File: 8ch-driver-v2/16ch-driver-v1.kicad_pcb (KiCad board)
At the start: 4 copper layers, 191.8 x 156.5 mm, 233 parts, among them J1 Barrel_Jack, Q1 2N7002E, Q10 2N7002E, Q11 2N7002E, Q12 2N7002E, Q13 2N7002E, Q14 2N7002E, Q15 2N7002E, Q16 2N7002E, Q2 2N7002E, Q3 2N7002E, Q4 2N7002E, Q5 2N7002E, Q6 2N7002E, Q7 2N7002E, Q8 2N7002E, Q9 2N7002E, U1 DRV104PWP, U10 DRV104PWP, U11 DRV104PWP, U12 DRV104PWP, U13 DRV104PWP, U14 DRV104PWP, U15 DRV104PWP, U16 DRV104PWP, U17 BD33FC0FP, U18 FT4232H MINI MODULE, U2 DRV104PWP, U3 DRV104PWP, U4 DRV104PWP, U5 DRV104PWP, U6 DRV104PWP, U7 DRV104PWP, U8 DRV104PWP, U9 DRV104PWP

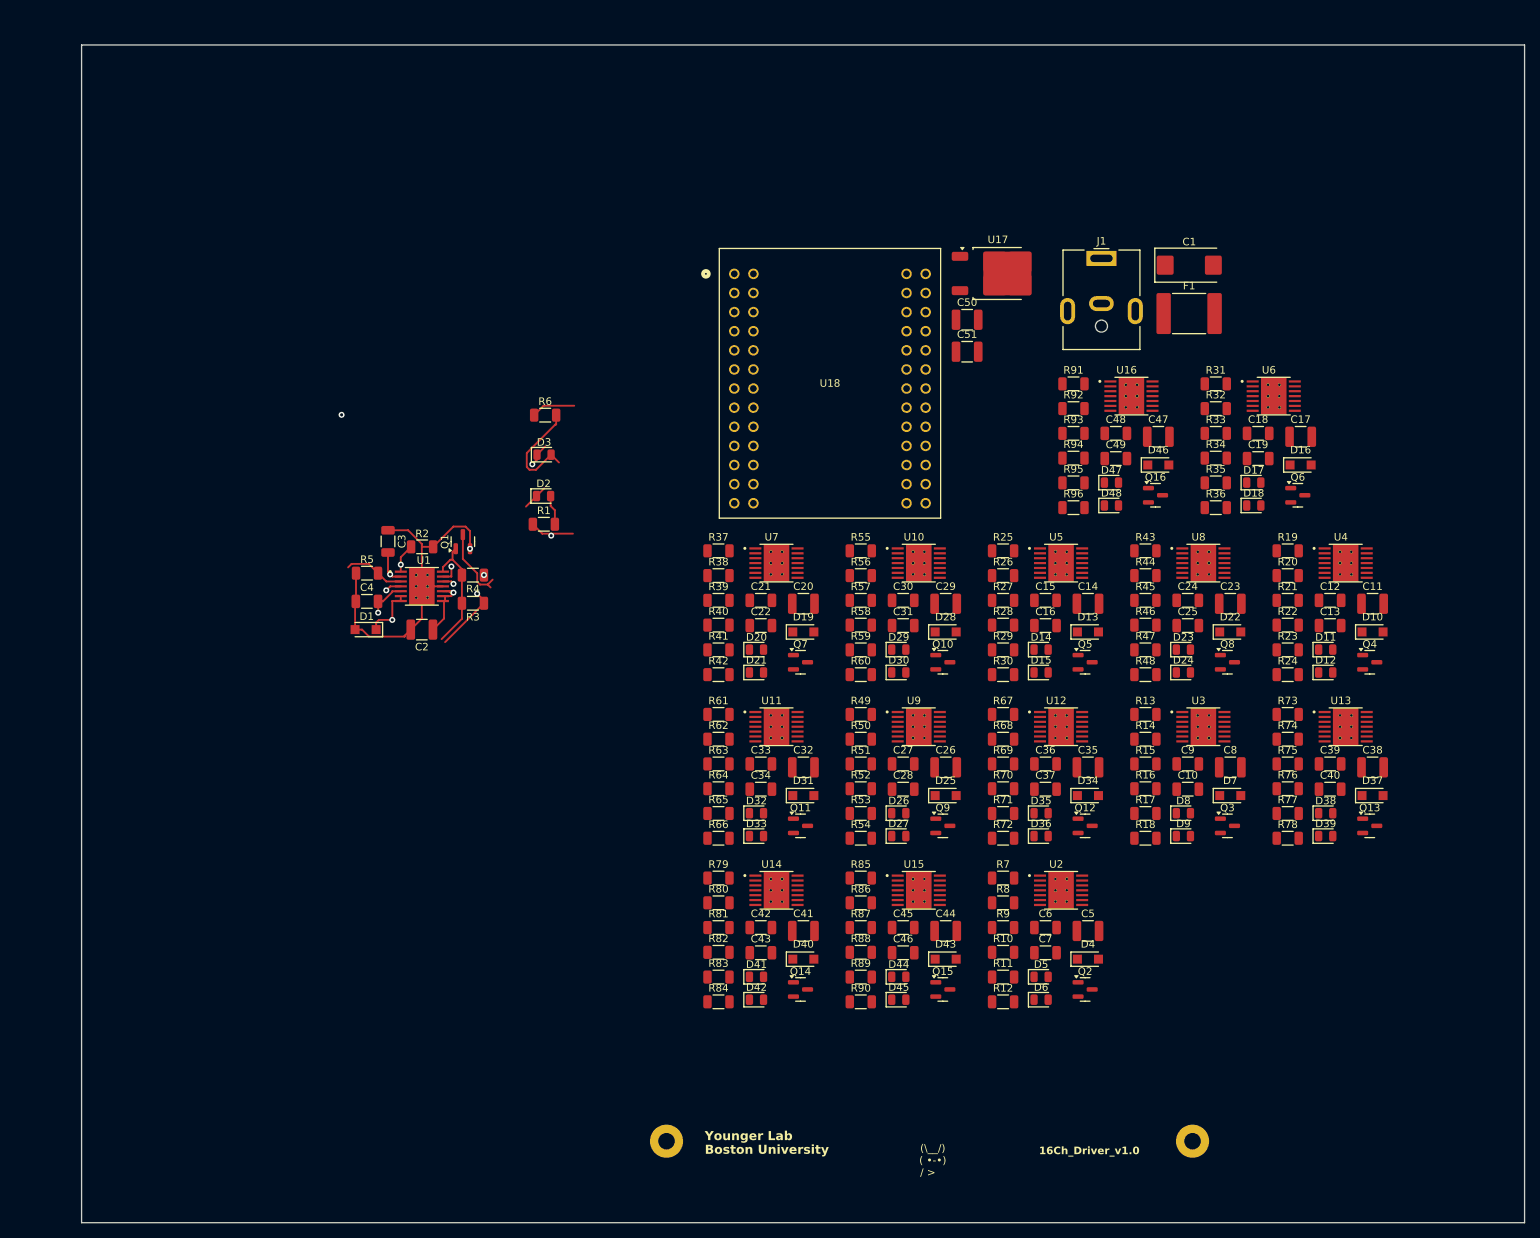
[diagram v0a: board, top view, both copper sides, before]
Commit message: push
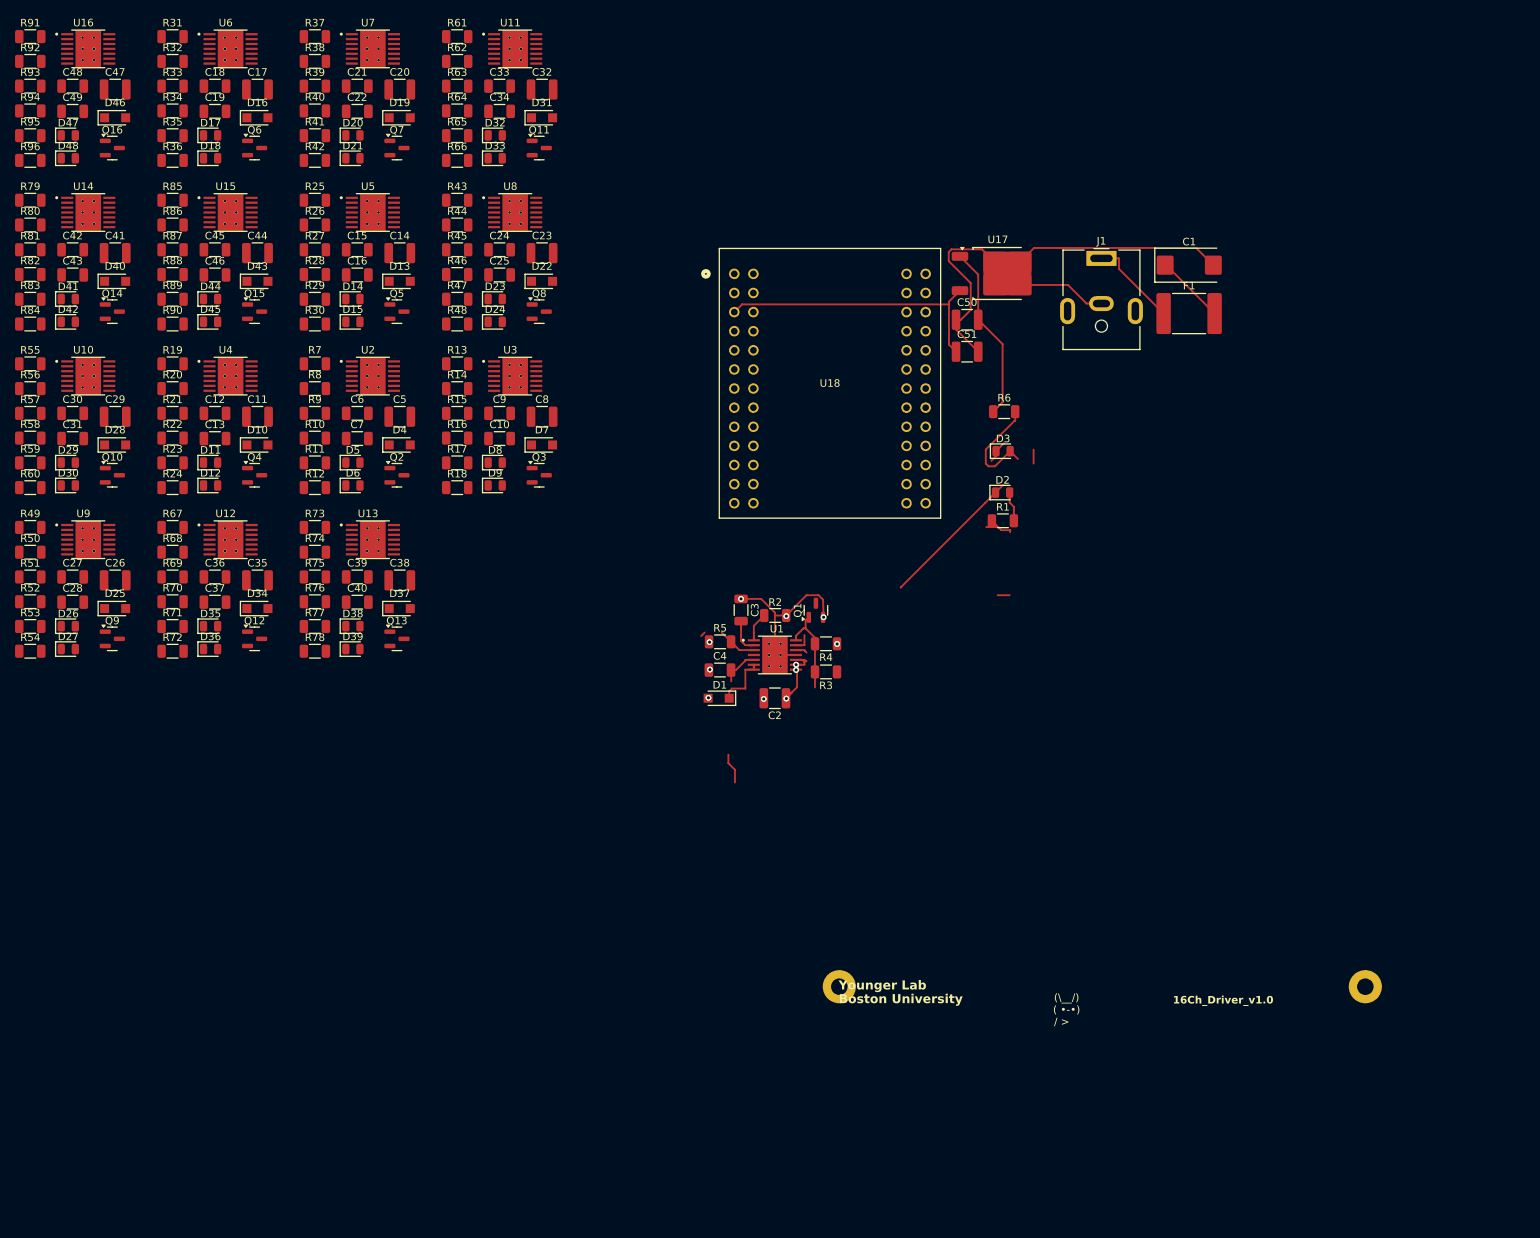
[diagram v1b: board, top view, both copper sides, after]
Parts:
- moved C11 150.2 mm to (46.4, 61.7)
- moved C12 150.2 mm to (40.7, 61.3)
- moved C13 150.2 mm to (40.7, 64.6)
- moved D10 150.2 mm to (46.4, 65.5)
- moved Q4 150.2 mm to (46.0, 69.5)
- moved R19 150.2 mm to (35.1, 54.7)
- moved R20 150.2 mm to (35.1, 58.0)
- moved R21 150.2 mm to (35.1, 61.3)
- moved R22 150.2 mm to (35.1, 64.5)
- moved R23 150.2 mm to (35.1, 67.8)
- moved R24 150.2 mm to (35.1, 71.1)
- moved U4 150.2 mm to (42.8, 56.3)
- moved D11 150.2 mm to (40.1, 67.8)
- moved D12 150.2 mm to (40.1, 70.8)
- moved C17 146.1 mm to (46.4, 18.2)
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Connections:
- net /SpikeAndHoldDriverAndLEDs-1/delay03 renamed /SpikeAndHoldDriverAndLEDs-1/delay
- net /SpikeAndHoldDriverAndLEDs-1/duty03 renamed /SpikeAndHoldDriverAndLEDs-1/duty
- net /SpikeAndHoldDriverAndLEDs-1/fault03 renamed /SpikeAndHoldDriverAndLEDs-1/fault
- net /SpikeAndHoldDriverAndLEDs-1/freq03 renamed /SpikeAndHoldDriverAndLEDs-1/freq
- net /SpikeAndHoldDriverAndLEDs-1/in_term03 renamed Net-(Q1-G)
- net /SpikeAndHoldDriverAndLEDs-10/delay03 renamed /SpikeAndHoldDriverAndLEDs-10/delay
- net /SpikeAndHoldDriverAndLEDs-10/duty03 renamed /SpikeAndHoldDriverAndLEDs-10/duty
- net /SpikeAndHoldDriverAndLEDs-10/fault03 renamed /SpikeAndHoldDriverAndLEDs-10/fault
- net /SpikeAndHoldDriverAndLEDs-10/freq03 renamed /SpikeAndHoldDriverAndLEDs-10/freq
- net /SpikeAndHoldDriverAndLEDs-10/in_term03 renamed Net-(Q10-G)
- net /SpikeAndHoldDriverAndLEDs-11/delay03 renamed /SpikeAndHoldDriverAndLEDs-11/delay
- net /SpikeAndHoldDriverAndLEDs-11/duty03 renamed /SpikeAndHoldDriverAndLEDs-11/duty
- net /SpikeAndHoldDriverAndLEDs-11/fault03 renamed /SpikeAndHoldDriverAndLEDs-11/fault
- net /SpikeAndHoldDriverAndLEDs-11/freq03 renamed /SpikeAndHoldDriverAndLEDs-11/freq
- net /SpikeAndHoldDriverAndLEDs-11/in_term03 renamed Net-(Q11-G)
- net /SpikeAndHoldDriverAndLEDs-12/delay03 renamed /SpikeAndHoldDriverAndLEDs-12/delay
- net /SpikeAndHoldDriverAndLEDs-12/duty03 renamed /SpikeAndHoldDriverAndLEDs-12/duty
- net /SpikeAndHoldDriverAndLEDs-12/fault03 renamed /SpikeAndHoldDriverAndLEDs-12/fault
- net /SpikeAndHoldDriverAndLEDs-12/freq03 renamed /SpikeAndHoldDriverAndLEDs-12/freq
- net /SpikeAndHoldDriverAndLEDs-12/in_term03 renamed Net-(Q12-G)
- net /SpikeAndHoldDriverAndLEDs-13/delay03 renamed /SpikeAndHoldDriverAndLEDs-13/delay
- net /SpikeAndHoldDriverAndLEDs-13/duty03 renamed /SpikeAndHoldDriverAndLEDs-13/duty
- net /SpikeAndHoldDriverAndLEDs-13/fault03 renamed /SpikeAndHoldDriverAndLEDs-13/fault
- net /SpikeAndHoldDriverAndLEDs-13/freq03 renamed /SpikeAndHoldDriverAndLEDs-13/freq
- net /SpikeAndHoldDriverAndLEDs-13/in_term03 renamed Net-(Q13-G)
- net /SpikeAndHoldDriverAndLEDs-14/delay03 renamed /SpikeAndHoldDriverAndLEDs-14/delay
- net /SpikeAndHoldDriverAndLEDs-14/duty03 renamed /SpikeAndHoldDriverAndLEDs-14/duty
- net /SpikeAndHoldDriverAndLEDs-14/fault03 renamed /SpikeAndHoldDriverAndLEDs-14/fault
- net /SpikeAndHoldDriverAndLEDs-14/freq03 renamed /SpikeAndHoldDriverAndLEDs-14/freq
- net /SpikeAndHoldDriverAndLEDs-14/in_term03 renamed Net-(Q14-G)
- net /SpikeAndHoldDriverAndLEDs-15/delay03 renamed /SpikeAndHoldDriverAndLEDs-15/delay
- net /SpikeAndHoldDriverAndLEDs-15/duty03 renamed /SpikeAndHoldDriverAndLEDs-15/duty
- net /SpikeAndHoldDriverAndLEDs-15/fault03 renamed /SpikeAndHoldDriverAndLEDs-15/fault
- net /SpikeAndHoldDriverAndLEDs-15/freq03 renamed /SpikeAndHoldDriverAndLEDs-15/freq
- net /SpikeAndHoldDriverAndLEDs-15/in_term03 renamed Net-(Q15-G)
- net /SpikeAndHoldDriverAndLEDs-16/delay03 renamed /SpikeAndHoldDriverAndLEDs-16/delay
- net /SpikeAndHoldDriverAndLEDs-16/duty03 renamed /SpikeAndHoldDriverAndLEDs-16/duty
- net /SpikeAndHoldDriverAndLEDs-16/fault03 renamed /SpikeAndHoldDriverAndLEDs-16/fault
- net /SpikeAndHoldDriverAndLEDs-16/freq03 renamed /SpikeAndHoldDriverAndLEDs-16/freq
- net /SpikeAndHoldDriverAndLEDs-16/in_term03 renamed Net-(Q16-G)
- net /SpikeAndHoldDriverAndLEDs-2/delay03 renamed /SpikeAndHoldDriverAndLEDs-2/delay
- net /SpikeAndHoldDriverAndLEDs-2/duty03 renamed /SpikeAndHoldDriverAndLEDs-2/duty
- net /SpikeAndHoldDriverAndLEDs-2/fault03 renamed /SpikeAndHoldDriverAndLEDs-2/fault
- net /SpikeAndHoldDriverAndLEDs-2/freq03 renamed /SpikeAndHoldDriverAndLEDs-2/freq
- net /SpikeAndHoldDriverAndLEDs-2/in_term03 renamed Net-(Q2-G)
- net /SpikeAndHoldDriverAndLEDs-3/delay03 renamed /SpikeAndHoldDriverAndLEDs-3/delay
- net /SpikeAndHoldDriverAndLEDs-3/duty03 renamed /SpikeAndHoldDriverAndLEDs-3/duty
- net /SpikeAndHoldDriverAndLEDs-3/fault03 renamed /SpikeAndHoldDriverAndLEDs-3/fault
- net /SpikeAndHoldDriverAndLEDs-3/freq03 renamed /SpikeAndHoldDriverAndLEDs-3/freq
- net /SpikeAndHoldDriverAndLEDs-3/in_term03 renamed Net-(Q3-G)
- net /SpikeAndHoldDriverAndLEDs-4/delay03 renamed /SpikeAndHoldDriverAndLEDs-4/delay
- net /SpikeAndHoldDriverAndLEDs-4/duty03 renamed /SpikeAndHoldDriverAndLEDs-4/duty
- net /SpikeAndHoldDriverAndLEDs-4/fault03 renamed /SpikeAndHoldDriverAndLEDs-4/fault
- net /SpikeAndHoldDriverAndLEDs-4/freq03 renamed /SpikeAndHoldDriverAndLEDs-4/freq
- net /SpikeAndHoldDriverAndLEDs-4/in_term03 renamed Net-(Q4-G)
- net /SpikeAndHoldDriverAndLEDs-5/delay03 renamed /SpikeAndHoldDriverAndLEDs-5/delay
- net /SpikeAndHoldDriverAndLEDs-5/duty03 renamed /SpikeAndHoldDriverAndLEDs-5/duty
- net /SpikeAndHoldDriverAndLEDs-5/fault03 renamed /SpikeAndHoldDriverAndLEDs-5/fault
- net /SpikeAndHoldDriverAndLEDs-5/freq03 renamed /SpikeAndHoldDriverAndLEDs-5/freq
- net /SpikeAndHoldDriverAndLEDs-5/in_term03 renamed Net-(Q5-G)
- net /SpikeAndHoldDriverAndLEDs-6/delay03 renamed /SpikeAndHoldDriverAndLEDs-6/delay
- net /SpikeAndHoldDriverAndLEDs-6/duty03 renamed /SpikeAndHoldDriverAndLEDs-6/duty
- net /SpikeAndHoldDriverAndLEDs-6/fault03 renamed /SpikeAndHoldDriverAndLEDs-6/fault
- net /SpikeAndHoldDriverAndLEDs-6/freq03 renamed /SpikeAndHoldDriverAndLEDs-6/freq
- net /SpikeAndHoldDriverAndLEDs-6/in_term03 renamed Net-(Q6-G)
- net /SpikeAndHoldDriverAndLEDs-7/delay03 renamed /SpikeAndHoldDriverAndLEDs-7/delay
- net /SpikeAndHoldDriverAndLEDs-7/duty03 renamed /SpikeAndHoldDriverAndLEDs-7/duty
- net /SpikeAndHoldDriverAndLEDs-7/fault03 renamed /SpikeAndHoldDriverAndLEDs-7/fault
- net /SpikeAndHoldDriverAndLEDs-7/freq03 renamed /SpikeAndHoldDriverAndLEDs-7/freq
- net /SpikeAndHoldDriverAndLEDs-7/in_term03 renamed Net-(Q7-G)
- net /SpikeAndHoldDriverAndLEDs-8/delay03 renamed /SpikeAndHoldDriverAndLEDs-8/delay
- net /SpikeAndHoldDriverAndLEDs-8/duty03 renamed /SpikeAndHoldDriverAndLEDs-8/duty
- net /SpikeAndHoldDriverAndLEDs-8/fault03 renamed /SpikeAndHoldDriverAndLEDs-8/fault
- net /SpikeAndHoldDriverAndLEDs-8/freq03 renamed /SpikeAndHoldDriverAndLEDs-8/freq
- net /SpikeAndHoldDriverAndLEDs-8/in_term03 renamed Net-(Q8-G)
- net /SpikeAndHoldDriverAndLEDs-9/delay03 renamed /SpikeAndHoldDriverAndLEDs-9/delay
- net /SpikeAndHoldDriverAndLEDs-9/duty03 renamed /SpikeAndHoldDriverAndLEDs-9/duty
- net /SpikeAndHoldDriverAndLEDs-9/fault03 renamed /SpikeAndHoldDriverAndLEDs-9/fault
- net /SpikeAndHoldDriverAndLEDs-9/freq03 renamed /SpikeAndHoldDriverAndLEDs-9/freq
- net /SpikeAndHoldDriverAndLEDs-9/in_term03 renamed Net-(Q9-G)
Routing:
- net GND: track 46.2 -> 101.3 mm, vias 2 -> 8
- net +3.3V: track 0.00 -> 38.1 mm
- net +12V: track 22.2 -> 48.4 mm, vias 2 -> 3
- net /12V_IN: track 0.00 -> 12.1 mm
- net /SpikeAndHoldDriverAndLEDs-1/TTLInput: track 8.96 -> 0.56 mm, vias 1 -> 0
- net Net-(D2-K): track 13.5 -> 21.4 mm
- net /SpikeAndHoldDriverAndLEDs-1/delay: track 11.5 -> 5.38 mm, vias 1 -> 0
- net (no net): track 0.00 -> 4.05 mm, vias 1 -> 0
- net Net-(Q1-G): track 16.1 -> 12.6 mm
- net Net-(D3-A): track 14.3 -> 16.9 mm
- net unconnected-(U1-MASTER-Pad4): track 2.15 -> 0.00 mm, vias 1 -> 0
- net Net-(D2-A): track 3.98 -> 5.58 mm
- net /SpikeAndHoldDriverAndLEDs-1/freq: track 8.16 -> 6.65 mm
- net unconnected-(U1-SYNC-Pad12): track 2.64 -> 1.57 mm, vias 1 -> 0
- net /SpikeAndHoldDriverAndLEDs-1/DriveOut: track 7.51 -> 8.30 mm, vias 1 -> 0
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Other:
- board outline removed
